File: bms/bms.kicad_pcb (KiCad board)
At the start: 8 copper layers, 60 x 60 mm, 62 parts, among them J2 3S pack power + cell-tap harn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, Q11 CSD18540Q5B reverse-pack FET A, Q12 CSD18540Q5B reverse-pack FET B, Q701 BSS138 pack protector latch r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, Q703 CSD18540Q5B BQ77915 discharge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, Q704 CSD18540Q5B BQ77915 charge FET, U11 LTC4368IMS-1 bidirectional pa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, U719 BQ7791500PWR autonomous 3S pr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

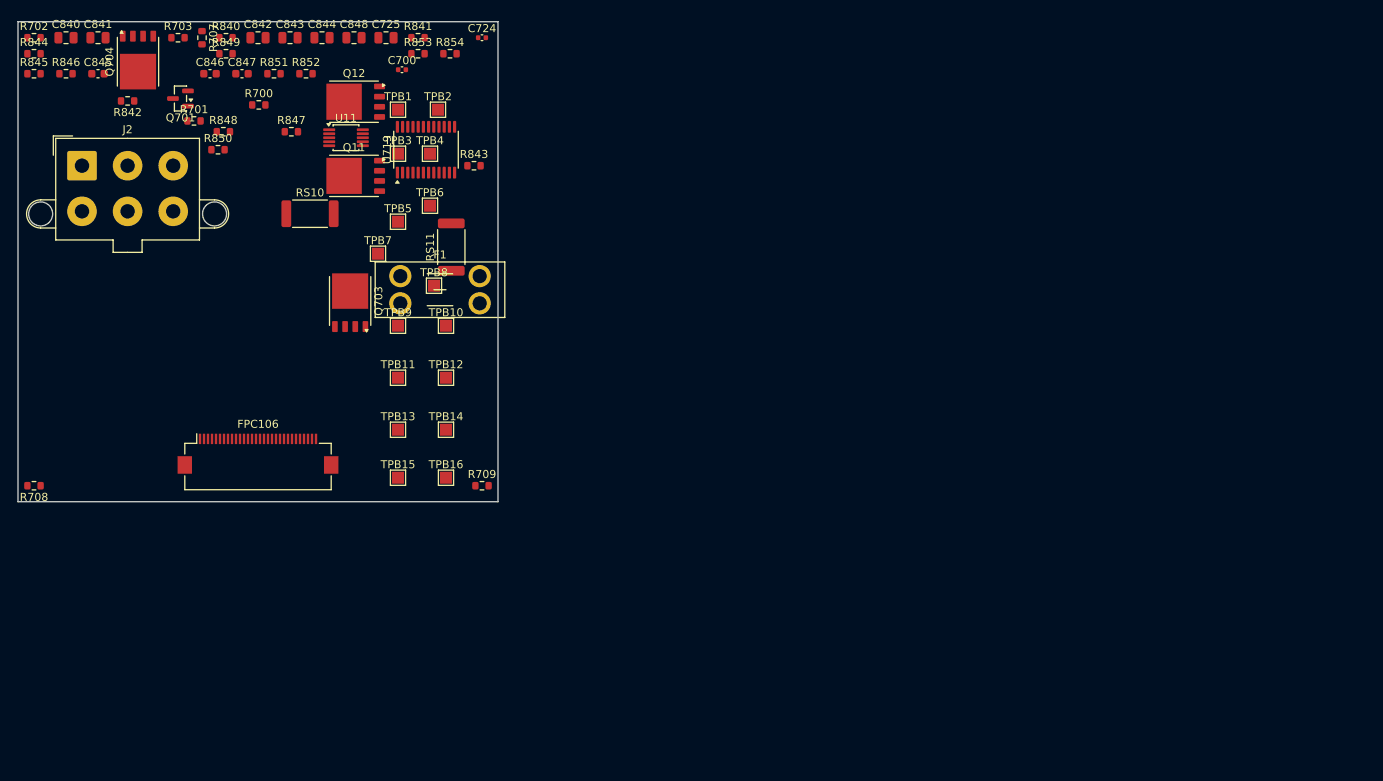
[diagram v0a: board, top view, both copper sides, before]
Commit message: finish the bms routing
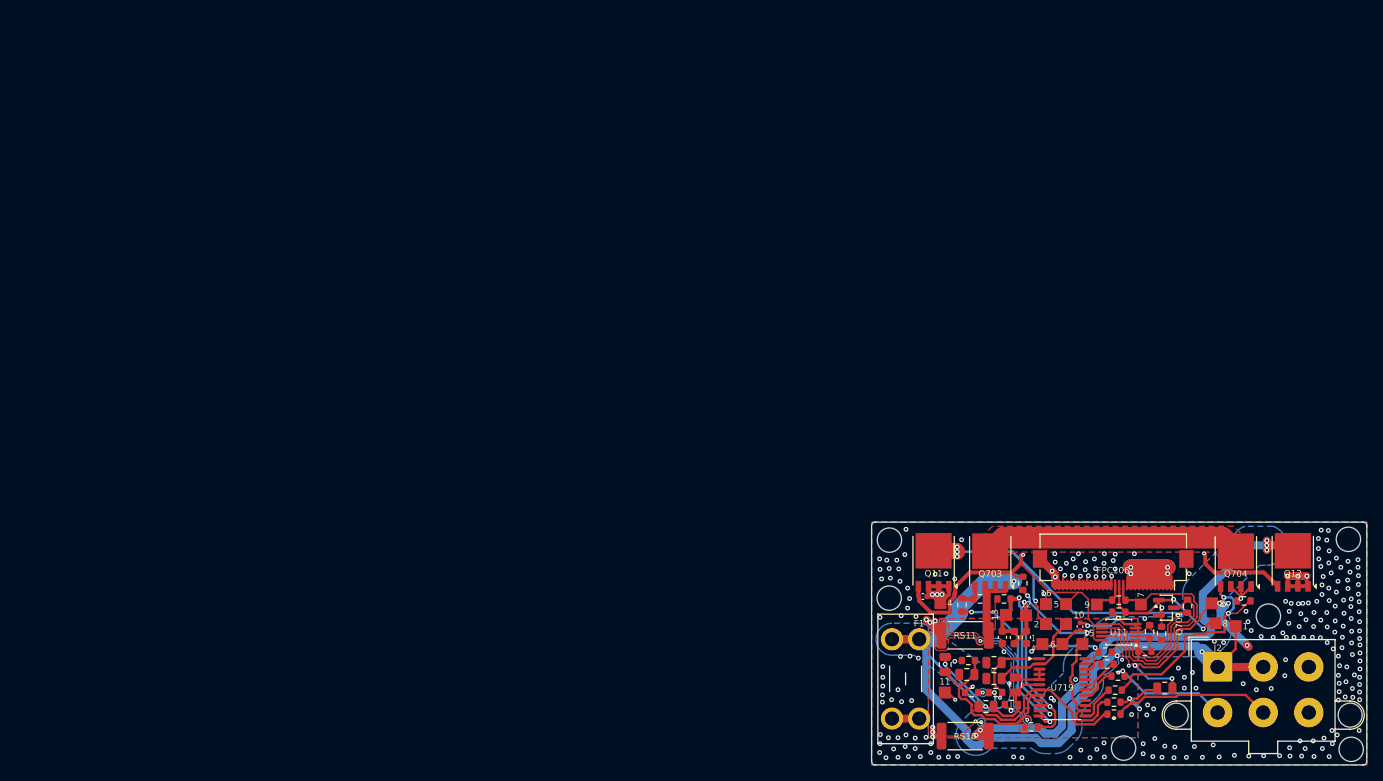
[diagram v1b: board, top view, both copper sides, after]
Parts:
- TPB1: value /PACK_POS_RAW -> PACK_POS_RAW
- TPB10: value /BMS_AVDD -> BMS_AVDD
- TPB11: value /BMS_VDD -> BMS_VDD
- TPB12: value /BMS_SRP -> BMS_SRP
- TPB13: value /BMS_SRN -> BMS_SRN
- TPB14: value /BMS_PRES -> BMS_PRES
- TPB15: value /BMS_LD -> BMS_LD
- TPB2: value /BAT_PROT_VIN -> BAT_PROT_VIN
- TPB3: value /PACK_POS_FUSED -> PACK_POS_FUSED
- TPB4: value /BAT_PROT_FET_COMMON -> BAT_PROT_FET_COMMON
- TPB5: value /BAT_PROT_GATE -> BAT_PROT_GATE
- TPB6: value /BAT_PROT_CGATE -> BAT_PROT_CGATE
- TPB7: value /PACK_FAULT_N -> PACK_FAULT_N
- TPB8: value /PACK_RETRY_PULSE -> PACK_RETRY_PULSE
- TPB9: value /MCU_3V3 -> MCU_3V3
- moved R702 159.4 mm to (142.9, 76.5), turned to 90 degrees
- moved J2 155.2 mm to (149.9, 80.7)
- moved Q704 150.8 mm to (152.2, 67.4), turned to -90 degrees
- moved R845 149.0 mm to (126.7, 88.2)
- moved R842 145.2 mm to (137.0, 86.5)
- moved R707 142.2 mm to (146.2, 73.0), turned to 90 degrees
- moved R844 141.8 mm to (119.2, 83.8), turned to 180 degrees
- moved R850 140.1 mm to (153.2, 72.4), turned to 180 degrees
- moved C840 139.8 mm to (122.0, 80.1), turned to 180 degrees
- moved Q701 138.7 mm to (143.5, 73.2), turned to 0 degrees
- moved C841 137.7 mm to (122.0, 82.1), turned to 180 degrees
- moved R708 136.4 mm to (137.6, 72.3), turned to 0 degrees
- moved C845 135.8 mm to (126.0, 77.0), turned to -90 degrees
- moved R701 135.4 mm to (141.4, 76.2), turned to 90 degrees
- moved R846 134.4 mm to (123.2, 72.2)
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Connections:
- F1 pad 2: /PACK_POS_FUSED -> /BAT_PROT_VIN
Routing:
- net /PACK_POS_RAW: track 0.00 -> 200.2 mm, vias 0 -> 7
- net /PACK_POS_FUSED: track 0.00 -> 154.2 mm, vias 0 -> 15
- net /BAT_PROT_SENSE: track 0.00 -> 151.4 mm, vias 0 -> 9
- net /BAT_PROT_VIN: track 0.00 -> 89.0 mm, vias 0 -> 5
- net /BAT_PROT_GATE: track 0.00 -> 75.9 mm, vias 0 -> 2
- net /BAT_PROT_FET_COMMON: track 0.00 -> 74.5 mm, vias 0 -> 6
- net /PACK_NEG_RAW: track 0.00 -> 60.5 mm, vias 0 -> 11
- net FG_VSS: track 0.00 -> 47.6 mm, vias 0 -> 237
- net /CELL2_TAP: track 0.00 -> 40.4 mm, vias 0 -> 1
- net /PACK_FAULT_N: track 0.00 -> 33.1 mm
- net /BMS_FET_COMMON: track 0.00 -> 32.1 mm
- net /BMS_VC1: track 0.00 -> 31.3 mm, vias 0 -> 2
- net /BMS_CHG_GATE: track 0.00 -> 28.0 mm, vias 0 -> 2
- net /BMS_SRP: track 0.00 -> 26.4 mm, vias 0 -> 2
- net /BMS_SRN: track 0.00 -> 24.7 mm, vias 0 -> 2
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- added copper zone on In2.Cu, net /BAT_PROT_FET_COMMON
- added copper zone on B.Cu, net /BAT_PROT_SENSE
- added copper zone on In1.Cu, net /BAT_PROT_VIN
- added copper zone on F.Cu, net /BMS_FET_COMMON
- added copper zone on B.Cu, net /PACK_NEG_RAW
- added copper zone on F.Cu, net /PACK_NEG_RAW
- added copper zone on In2.Cu, net /PACK_NEG_RAW
- added copper zone on In1.Cu, net /PACK_POS_FUSED
- added copper zone on B.Cu, net /PACK_POS_RAW
- added copper zone on In1.Cu, net /PACK_POS_RAW
- added copper zone on B.Cu, net FG_VSS
- added copper zone on F.Cu, net FG_VSS
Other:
- board size 60 x 60 mm -> 61.9 x 30.3 mm
- copper layers 8 -> 4
